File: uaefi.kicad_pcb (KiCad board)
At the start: 4 copper layers, 100 x 100 mm, 157 parts, among them J1 Conn_02x02_Odd_Even, J10 5569-16A2, J11 Conn_02x02_Odd_Even, J12 Conn_02x02_Odd_Even, J13 Conn_02x02_Odd_Even, J14 Conn_02x02_Odd_Even, J15 Conn_02x02_Odd_Even, J16 Conn_02x02_Odd_Even, J17 Conn_02x02_Odd_Even, J18 Conn_02x02_Odd_Even, J19 Conn_02x02_Odd_Even, J2 5569-20A2, J20 Conn_02x02_Odd_Even, J21 Conn_02x02_Odd_Even, J22 Conn_02x02_Odd_Even, J24 Conn_02x02_Odd_Even, J3 5569-06A2, J4 5569-08A2, J5 5569-18A2, J6 Conn_01x06, J7 Conn_01x05_Male, J8 USB_B_Mini, J9 USB_C, M1 Module-power_12and5V-0.2, M2 Module-knock-0.2, M3 Module-vr-discrete-0.5, M4 Module-vr-max9924-0.1, M5 Module-wbo-0.5, M6 Module:mega-mcu100/0.3, M7 Module-can-0.1, P1 Pad, P15 Pad, P16 Pad, P17 Pad, P18 Pad, P2 Pad, P3 Pad, P4 Pad, P7 Pad, P8 Pad, Q10 ISL9V3040D3ST, Q11 ISL9V3040D3ST, Q12 ISL9V3040D3ST, Q7 ISL9V3040D3ST, Q8 ISL9V3040D3ST, Q9 ISL9V3040D3ST, U1 TLE9201SG, U10 VNLD5160TR-E, U11 VNLD5160TR-E, U2 TLE9201SG, U3 MPX4/MPXH6400_MAP, U4 MAX31855KASA, U5 JDY-33, U6 VNLD5160TR-E, U7 VNLD5160TR-E, U8 VNLD5160TR-E, U9 VNLD5160TR-E

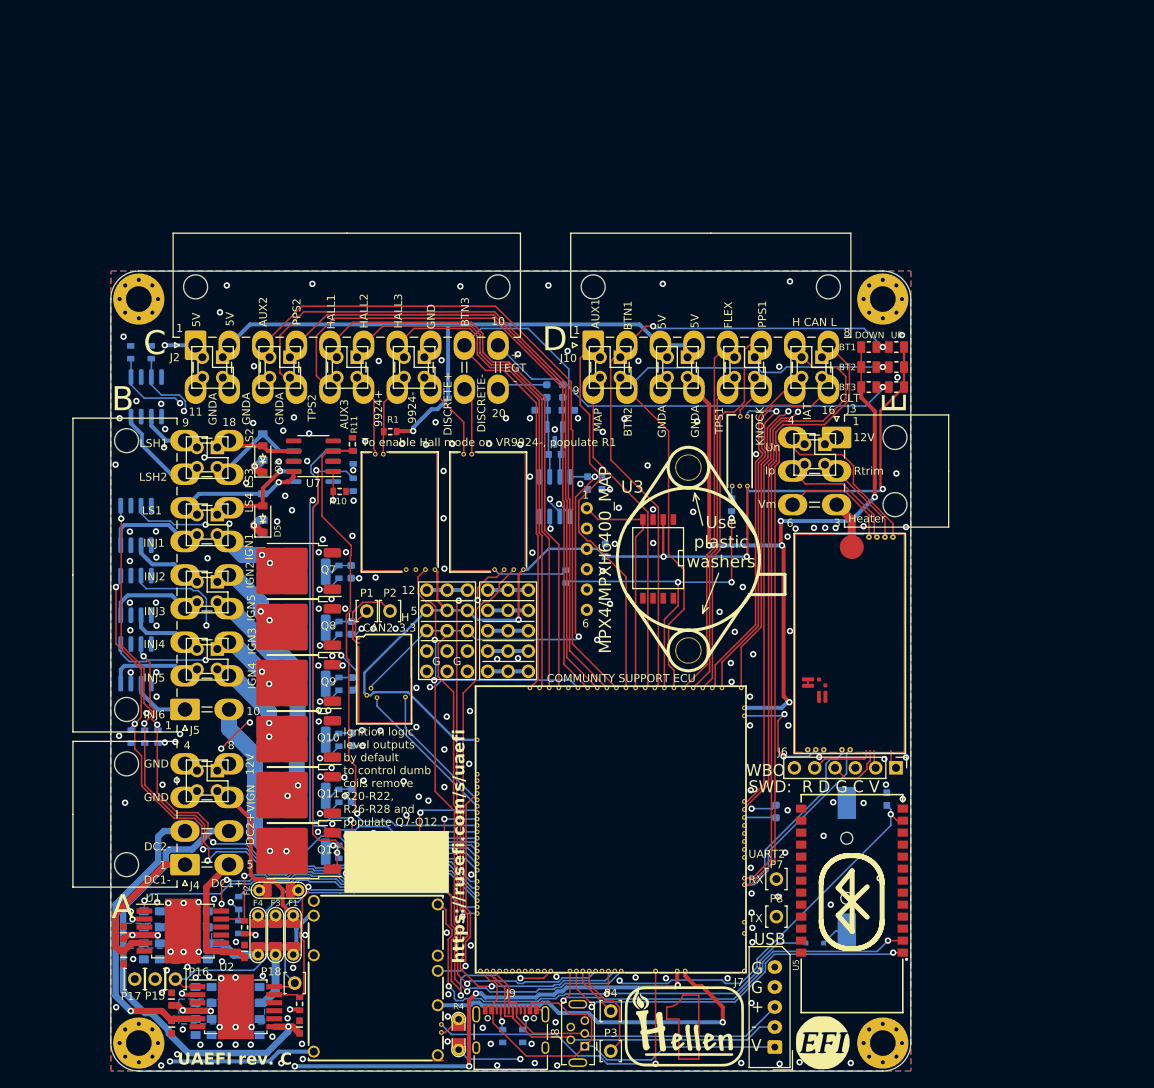
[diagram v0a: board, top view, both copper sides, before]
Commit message: Rev.D
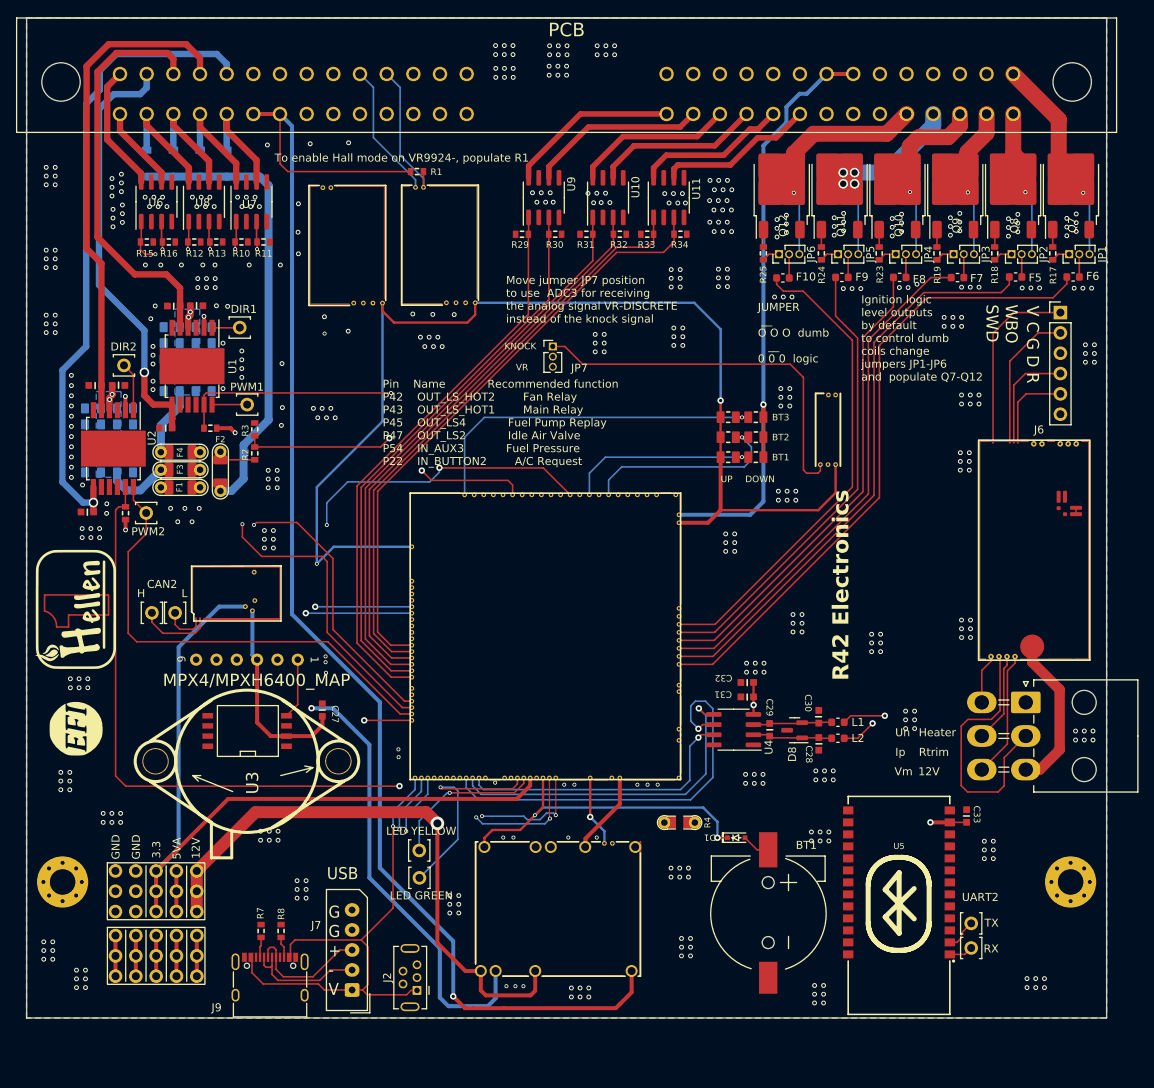
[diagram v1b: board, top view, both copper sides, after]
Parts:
- removed H3, H4: M3, MountingHole:MountingHole_3.2mm_M3_Pad_Via
- removed J10: 5569-16A2, Connector_Molex:Molex_Mini-Fit_Jr_5569-16A2_2x08_P4.20mm_Horizontal
- removed J11, J12, J13, J14, J15, J16, J17, J18, J19, J20, J21, J22, J24: Conn_02x02_Odd_Even, Connector_PinSocket_2.54mm:PinSocket_2x02_P2.54mm_Vertical
- removed J4: 5569-08A2, Connector_Molex:Molex_Mini-Fit_Jr_5569-08A2_2x04_P4.20mm_Horizontal
- removed J5: 5569-18A2, Connector_Molex:Molex_Mini-Fit_Jr_5569-18A2_2x09_P4.20mm_Horizontal
- removed J8: USB_B_Mini, hellen-one-common:USB-MINI-B-VERTICAL
- removed R20, R21, R22, R26, R27, R28: 0, Resistor_SMD:R_2512_6332Metric
- removed R5, R6: 0, hellen-one-common:R0603
- added G***: LOGO, kicad6-libraries:R42_Logo, F.Cu at (149.3, 99.2)
- added JP1: Jumper_3_Open, Connector_PinHeader_1.27mm:PinHeader_1x03_P1.27mm_Vertical, F.Cu at (169.8, 57.9)
- added JP2: Jumper_3_Open, Connector_PinHeader_1.27mm:PinHeader_1x03_P1.27mm_Vertical, F.Cu at (162.6, 57.9)
- added JP3: Jumper_3_Open, Connector_PinHeader_1.27mm:PinHeader_1x03_P1.27mm_Vertical, F.Cu at (155.4, 57.9)
- added JP4: Jumper_3_Open, Connector_PinHeader_1.27mm:PinHeader_1x03_P1.27mm_Vertical, F.Cu at (148.1, 57.9)
- added JP5: Jumper_3_Open, Connector_PinHeader_1.27mm:PinHeader_1x03_P1.27mm_Vertical, F.Cu at (140.9, 57.9)
- added JP6: Jumper_3_Open, Connector_PinHeader_1.27mm:PinHeader_1x03_P1.27mm_Vertical, F.Cu at (133.5, 57.9)
- added JP7: Jumper_3_Open, Connector_PinHeader_1.27mm:PinHeader_1x03_P1.27mm_Vertical, F.Cu at (105.3, 69.4)
- BT1, C27, C28, C29, C30, C31, C32, C33, D1, D8, F10, F5, F6, F7, F8, F9, L1, L2, R12, R13, R15, R16, R17, R18, R19, R2, R23, R24, R25, R29, R3, R30, R31, R32, R33, R34, R7, R8, U10, U11, U4, U6, U8, U9: moved to F.Cu
- D3, D5: moved to B.Cu
- J1: value Conn_02x02_Odd_Even -> 211PL562L0011; footprint Connector_PinSocket_2.54mm:PinSocket_2x02_P2.54mm_Vertical -> uaefi-main:211PL562L0011_2
- J2: value 5569-20A2 -> USB_B_Mini; footprint Connector_Molex:Molex_Mini-Fit_Jr_5569-20A2_2x10_P4.20mm_Horizontal -> hellen-one-common:USB-MINI-B-VERTICAL
- moved H2 118.2 mm to (170.0, 136.4)
- moved Q7 108.4 mm to (170.0, 49.8), turned to 90 degrees
- moved Q8 105.4 mm to (162.8, 49.8), turned to 90 degrees
- moved Q9 103.4 mm to (155.6, 49.8), turned to 90 degrees
- moved Q12 102.9 mm to (133.9, 49.8), turned to 90 degrees
- moved Q10 102.2 mm to (148.3, 49.8), turned to 90 degrees
- moved Q11 102.1 mm to (141.1, 49.8), turned to 90 degrees
- moved G1 101.2 mm to (45.7, 117.2), turned to 90 degrees
- moved R17 97.7 mm to (167.7, 57.8), turned to -90 degrees
- moved F6 97.5 mm to (170.3, 60.7), turned to 180 degrees
- moved R18 94.4 mm to (160.5, 57.8), turned to -90 degrees
- moved F5 93.9 mm to (163.1, 60.7), turned to 180 degrees
- moved G2 92.6 mm to (45.7, 102.0), turned to 90 degrees
- moved R19 92.1 mm to (153.3, 57.8), turned to -90 degrees
- moved R25 91.7 mm to (131.6, 57.8), turned to -90 degrees
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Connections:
- F10 pad 1: Net-(F10-Pad1) -> Net-(JP6-C)
- F5 pad 1: Net-(F5-Pad1) -> Net-(JP2-C)
- F6 pad 1: Net-(F6-Pad1) -> Net-(JP1-C)
- F7 pad 1: Net-(F7-Pad1) -> Net-(JP3-C)
- F8 pad 1: Net-(F8-Pad1) -> Net-(JP4-C)
- F9 pad 1: Net-(F9-Pad1) -> Net-(JP5-C)
- J2 pad 1: +5VP -> /VBUS
- J2 pad 2: +5VP -> /USB-
- J2 pad 3: /IN_AUX2 -> /USB+
- J2 pad 4: /IN_PPS2 -> unconnected-(J2-ID-Pad4)
- J2 pad 5: /IN_HALL1 -> GND
- J2 pad 6: /IN_HALL2 -> GND
- R17 pad 2: Net-(F6-Pad1) -> Net-(JP1-A)
- R18 pad 2: Net-(F5-Pad1) -> Net-(JP2-A)
- R19 pad 2: Net-(F7-Pad1) -> Net-(JP3-A)
- R23 pad 2: Net-(F8-Pad1) -> Net-(JP4-A)
- R24 pad 2: Net-(F9-Pad1) -> Net-(JP5-A)
- R25 pad 2: Net-(F10-Pad1) -> Net-(JP6-A)
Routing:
- net /EGT-: track 6.33 -> 99.4 mm, vias 0 -> 1
- net /EGT+: track 10.1 -> 102.3 mm, vias 0 -> 1
- net /IN_VIGN: track 6.27 -> 95.2 mm, vias 0 -> 1
- net Net-(F10-Pad1): track 84.5 -> 0.00 mm, vias 2 -> 0
- net +5VA: track 171.1 -> 249.8 mm, vias 6 -> 2
- net GNDA: track 155.8 -> 78.4 mm, vias 5 -> 1
- net /12V_KEY: track 19.3 -> 90.9 mm
- net /EGT/SPI_SO: track 104.7 -> 35.8 mm
- net /EGT/SPI_SCK: track 107.3 -> 42.4 mm
- net +12V: track 25.7 -> 87.8 mm
- net /EGT/SPI_CS: track 111.5 -> 51.2 mm
- net /IGN6: track 3.97 -> 60.3 mm
- net /IN_KNOCK: track 1.56 -> 47.7 mm
- net /IN_KNOCK_RAW: track 4.49 -> 44.2 mm
- net /OUT_DC1+: track 17.1 -> 53.8 mm, vias 0 -> 1
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- added copper zone on B.Cu, net /OUT_IGN5
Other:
- board size 100 x 100 mm -> 135 x 125 mm
- board text added: "5VA"
- board text added: "DIR1"
- board text added: "DIR2"
- board text added: "DIS+"
- board text added: "DIS-"
- board text added: "Ignition logic level outputs by default to control dumb coils change jumpers JP1-JP6 and populate Q7-Q12"
- board text added: "JUMPER __ O O O dumb __ 0 0 0 logic"
- board text added: "KNOCK VR"
- board text added: "LED GREEN"
- board text added: "LED YELLOW"
- board text added: "Move jumper JP7 position to use ADC3 for receiving the analog signal VR-DISCRETE instead of the knock signal"
- board text added: "PWM1"
- board text added: "PWM2"
- board text added: "Pin Name Recommended function P42 OUT_LS_HOT2 Fan Relay P43 OUT_LS_HOT1 Main Relay P45 OUT_LS4 Fuel Pump Replay P47 OUT_LS2 Idle Air Valve P54 IN_AUX3 Fuel Pressure P22 IN_BUTTON2 A/C Request"
- board text added: "R42 Electronics"
- board text added: "UART2 TX RX"
- board text added: "V C G D R"
- board text added: "WBO SWD"
- board text removed: "1"
- board text removed: "10"
- board text removed: "11"
- board text removed: "12"
- board text removed: "16"
- board text removed: "18"
- board text removed: "20"
- board text removed: "3"
- board text removed: "4"
- board text removed: "5"
- board text removed: "6"
- board text removed: "8"
- board text removed: "9"
- board text removed: "A"
- board text removed: "B"
- board text removed: "C"
- board text removed: "COMMUNITY SUPPORT ECU"
- board text removed: "D"
- board text removed: "DISCRETE+"
- board text removed: "DISCRETE-"
- board text removed: "E"
- board text removed: "G"
- board text removed: "H CAN L"
- board text removed: "Ignition logic level outputs by default to control dumb coils remove R20-R22, R26-R28 and populate Q7-Q12"
- board text removed: "SWD: R D G C V"
- board text removed: "UAEFI rev. C"
- board text removed: "UART2 RX TX"
- board text removed: "WBO"
- board text removed: "https://rusefi.com/s/uaefi"
